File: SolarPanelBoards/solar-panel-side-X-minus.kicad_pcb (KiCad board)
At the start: 2 copper layers, 82 x 99 mm, 24 parts, among them J1 Conn_01x06, U1 OPT3001DNPT

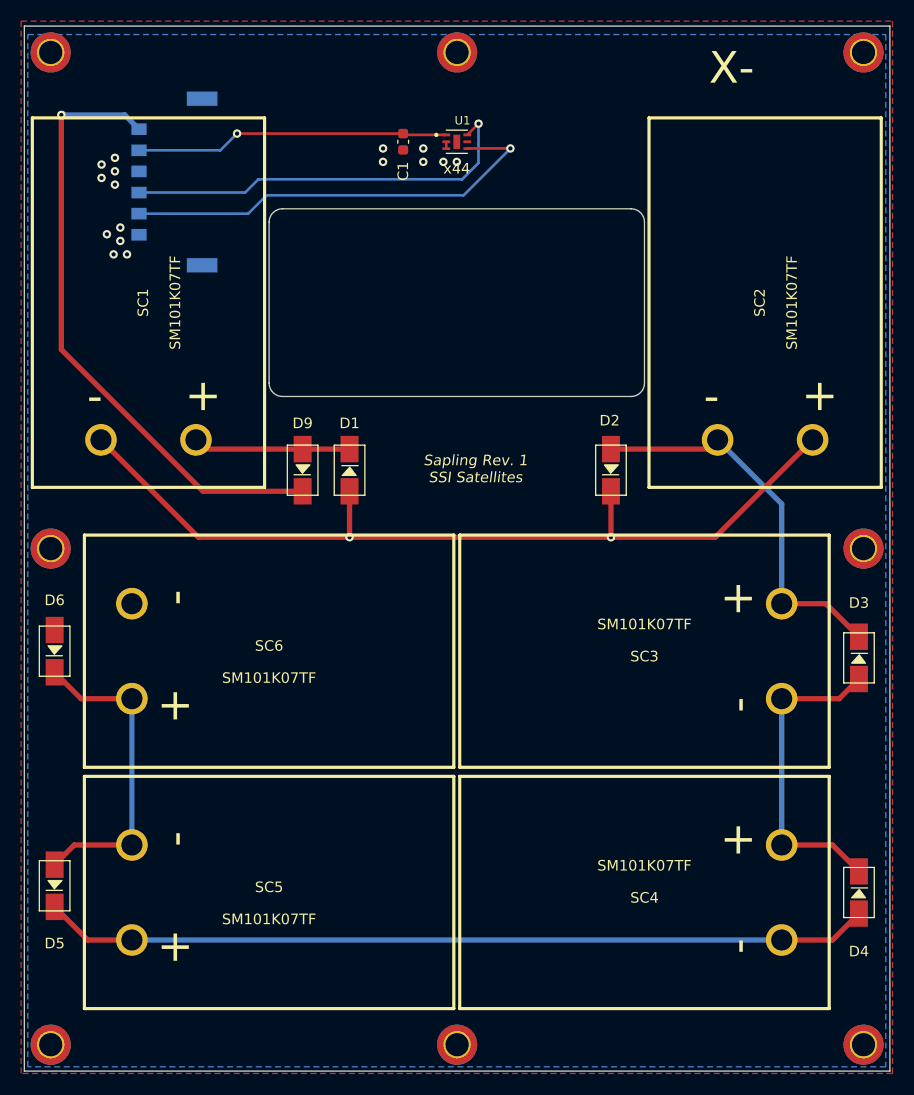
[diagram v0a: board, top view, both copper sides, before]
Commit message: rearranged x-minus
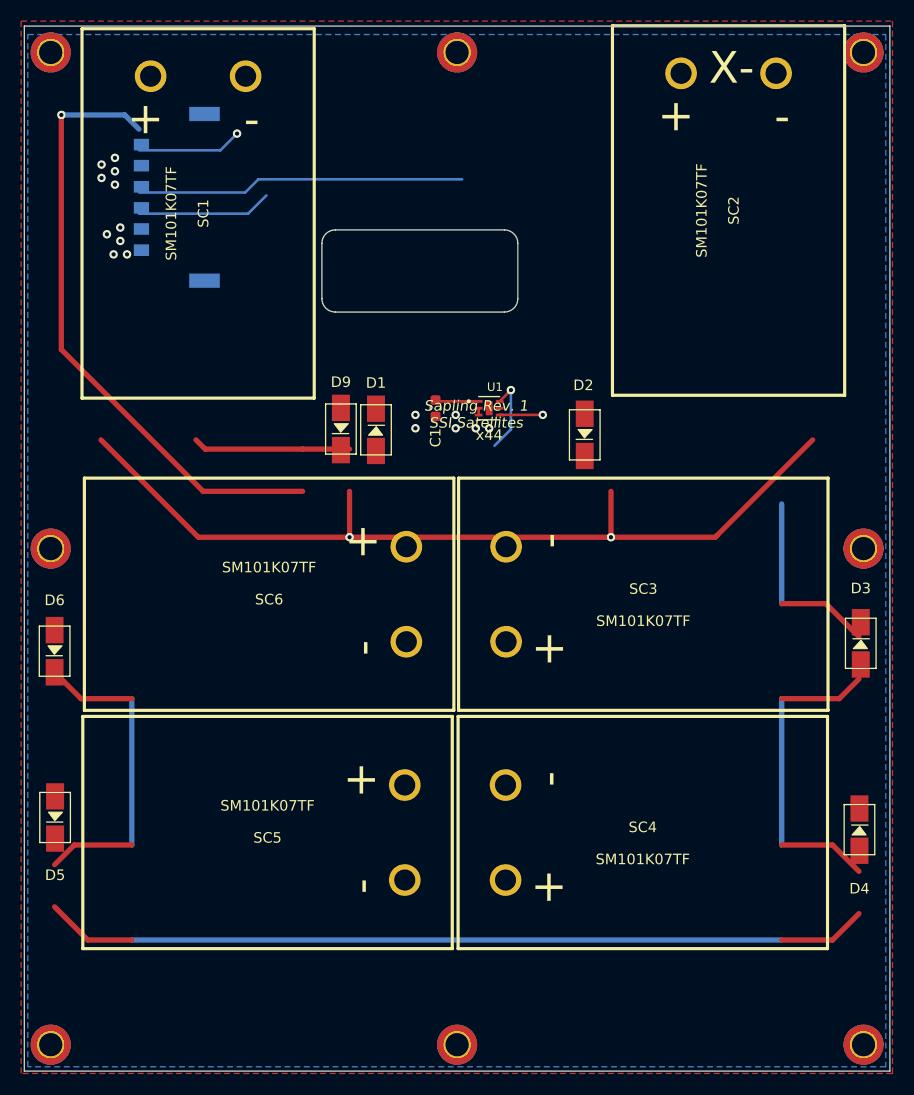
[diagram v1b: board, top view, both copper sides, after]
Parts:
- moved C1 25.4 mm to (149.1, 79.8)
- moved U1 25.4 mm to (154.2, 79.8)
- moved SC1 9.67 mm to (126.6, 61.4), turned to 90 degrees
- moved SC2 9.39 mm to (176.9, 61.1), turned to 90 degrees
- moved D5 6.47 mm to (113.1, 118.6)
- moved D4 5.96 mm to (189.3, 119.8)
- moved SC4 5.68 mm to (168.8, 120.0), turned to 180 degrees
- moved SC5 5.68 mm to (133.2, 120.0), turned to 0 degrees
- moved SC3 5.40 mm to (168.8, 97.5), turned to 180 degrees
- moved SC6 5.40 mm to (133.3, 97.5), turned to 0 degrees
- moved D9 5.32 mm to (140.2, 81.8)
- moved D1 4.57 mm to (143.5, 81.9)
- moved D2 4.17 mm to (163.2, 82.4)
- moved J1 1.47 mm to (124.8, 59.9)
- moved D3 1.39 mm to (189.4, 102.1)
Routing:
- net Net-(D4-Pad2): track 78.5 -> 17.0 mm
- net Net-(D3-Pad2): track 30.3 -> 91.9 mm
- net SCL: track 42.0 -> 4.28 mm
- net GND: track 0.65 -> 31.8 mm, vias 16 -> 12
- net +3V3: track 29.9 -> 4.14 mm, vias 1 -> 0
- net VSOLAR: track 58.8 -> 83.8 mm, vias 1 -> 2
- net Net-(D2-Pad2): track 37.1 -> 18.1 mm
- net SDA: track 38.6 -> 20.2 mm
- net Net-(D1-Pad1): track 14.9 -> 0.00 mm, vias 0 -> 4
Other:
- outline, holes or cut-outs redrawn
- net class Default removed
